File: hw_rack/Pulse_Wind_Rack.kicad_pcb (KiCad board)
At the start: 2 copper layers, 21 x 22 mm, 12 parts, among them J1 PH2.00, J2 PH2.00, J3 AudioJack4, U1 ME6206A33XG

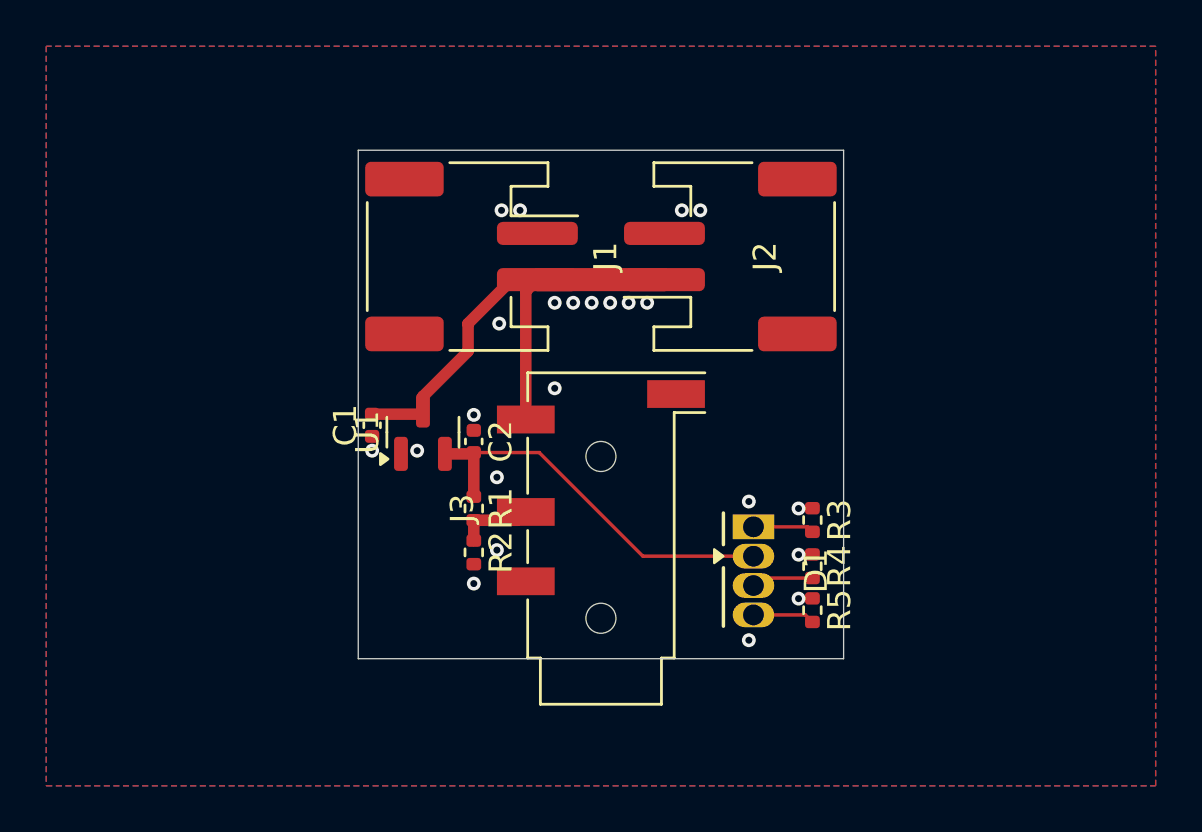
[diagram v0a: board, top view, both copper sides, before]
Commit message: hw: Finalize rack board design
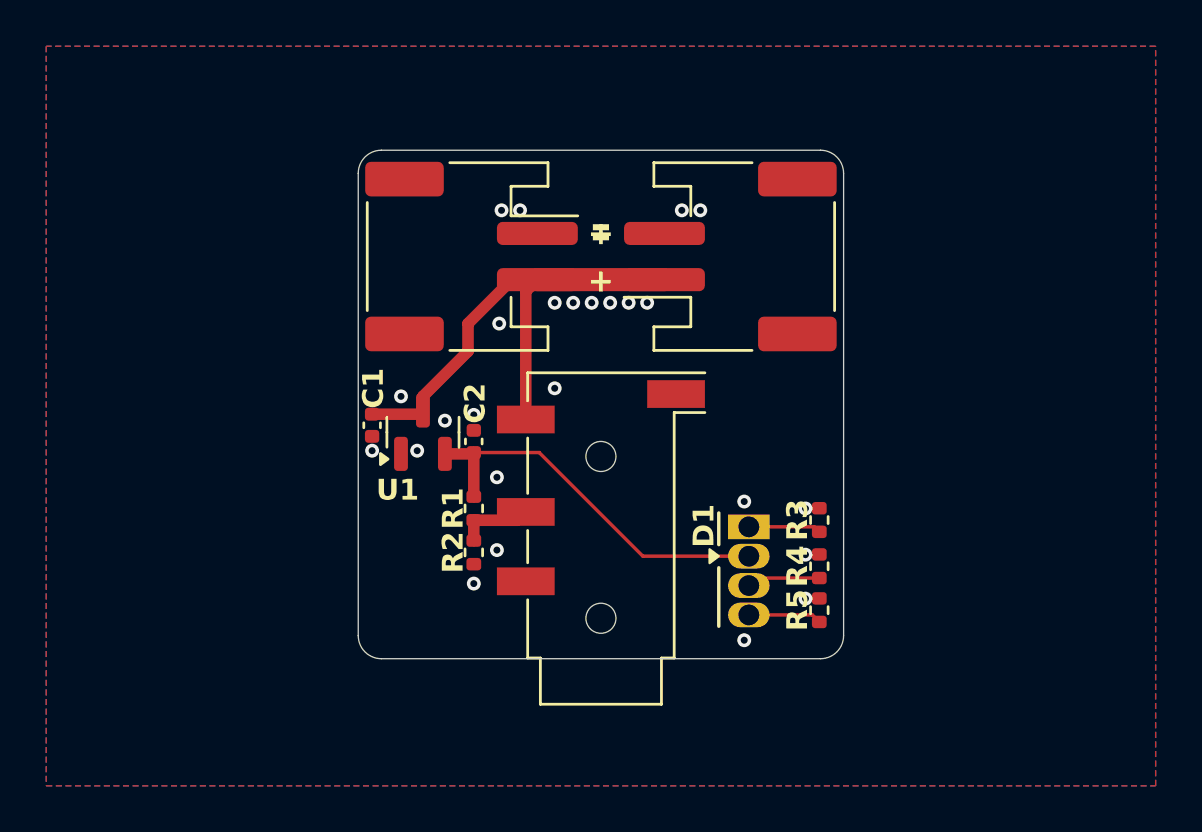
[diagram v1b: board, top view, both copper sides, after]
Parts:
- added G***: LOGO, LOGO, B.Cu at (152.8, 87.3)
- added G***: LOGO, LOGO, B.Cu at (157.8, 87.1)
- moved R3 0.30 mm to (159.4, 100.5)
- moved R4 0.30 mm to (159.4, 102.5)
- moved R5 0.30 mm to (159.4, 104.4)
- moved D1 0.20 mm to (156.4, 100.8)
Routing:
- net GND: vias 23 -> 25
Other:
- outline, holes or cut-outs redrawn
- board text added: "+"
- board text added: "<25-"
- board text added: ">"
- board text added: "Rev. 1"
- board text added: "大暑"
